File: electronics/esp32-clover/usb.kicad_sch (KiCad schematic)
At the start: 23 parts, among them J1 USB4055-30-A, Q2 MMDT3904, U2 CP2102N-Axx-xQFN20

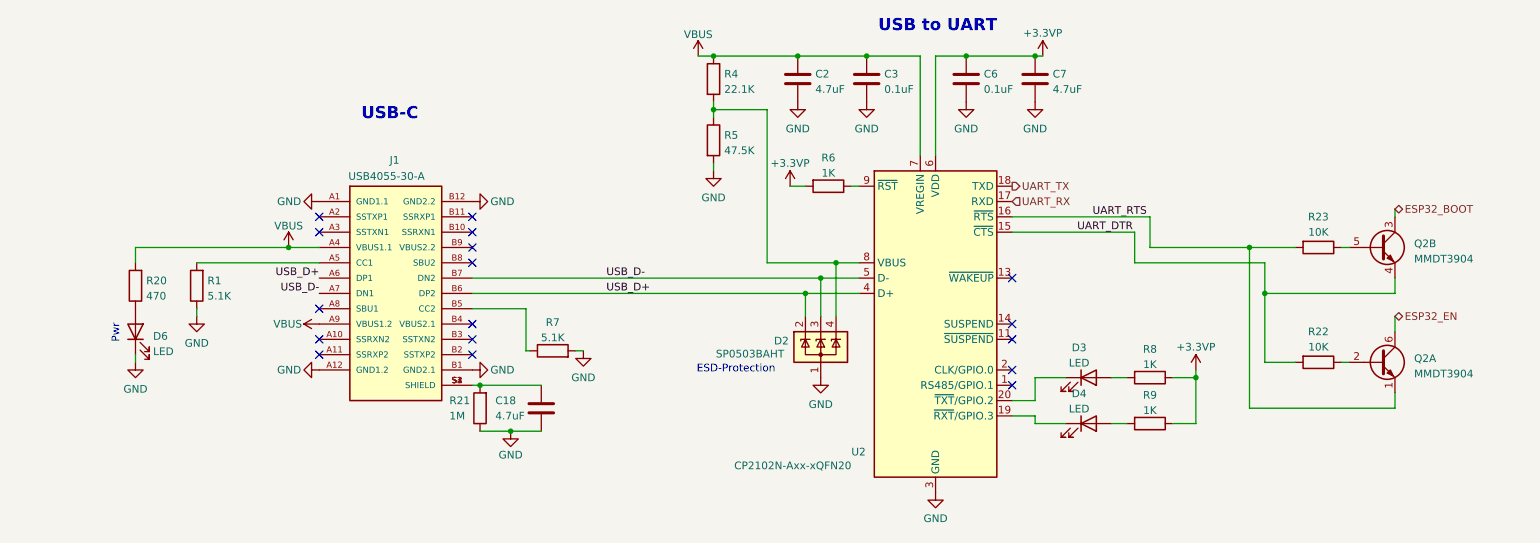
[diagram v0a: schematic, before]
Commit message: update before switching to stm32
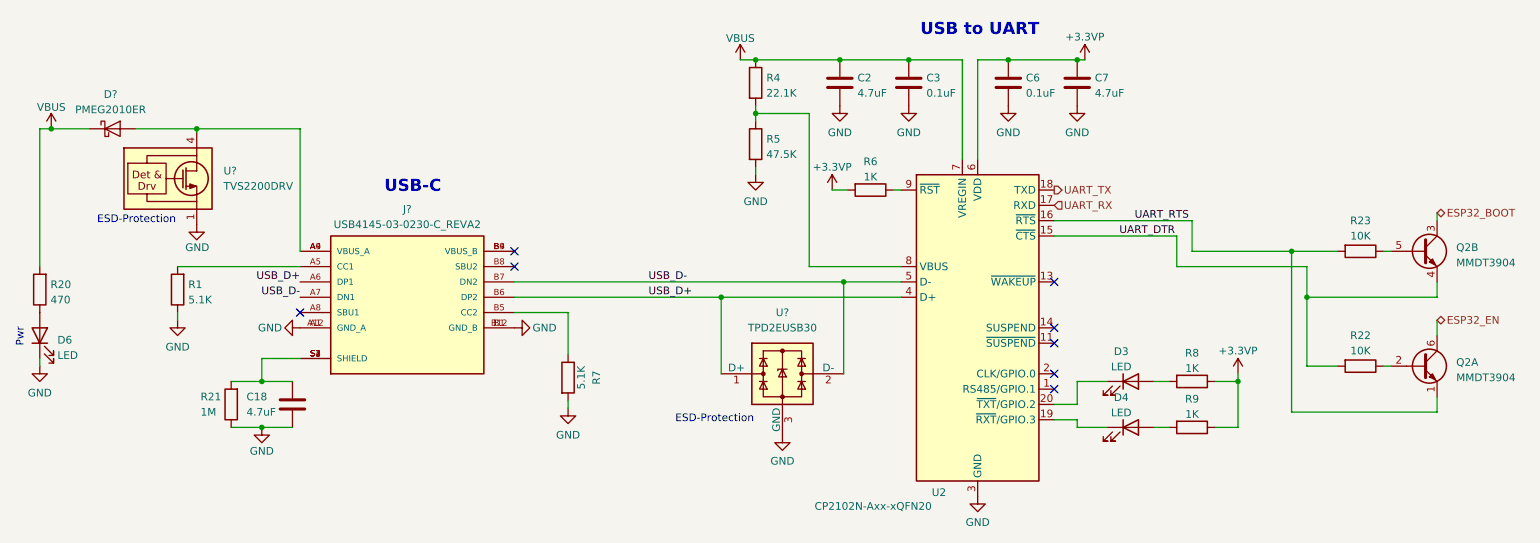
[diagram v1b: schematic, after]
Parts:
- removed D2: SP0503BAHT, Package_TO_SOT_SMD:SOT-143, symbol Power_Protection:SP0503BAHT
- removed J1: USB4055-30-A, USB4055-30-A:USB4055-30-A, symbol USB4055-30-A:USB4055-30-A
- added D?: PMEG2010ER, Diode_SMD:Nexperia_CFP3_SOD-123W, symbol Diode:PMEG2010ER
- added J?: USB4145-03-0230-C_REVA2, connectors_usb:USB4145-03-0230-C_REVA2, symbol connectors_usb:USB4145-03-0230-C_REVA2
- added U?: TVS2200DRV, Package_SON:WSON-6-1EP_2x2mm_P0.65mm_EP1x1.6mm, symbol Power_Protection:TVS2200DRV
- added U?: TPD2EUSB30, Package_TO_SOT_SMD:Texas_DRT-3, symbol Power_Protection:TPD2EUSB30
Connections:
- net GND: now also J?.A1 (GND_A), J?.A12 (GND_A), J?.B1 (GND_B), J?.B12 (GND_B), U?.1 (GND), U?.2 (GND), U?.3 (GND), U?.3 (GND), U?.7 (GND)
- net USB_D+: now also J?.A6 (DP1), J?.B6 (DP2), U?.1 (D+)
- net USB_D-: now also J?.A7 (DN1), J?.B7 (DN2), U?.2 (D-)
- net VBUS: now also D?.1 (K)
- net at C18.1, R21.2: now also J?.S1 (SHIELD), J?.S2 (SHIELD), J?.S3 (SHIELD), J?.S4 (SHIELD)
- net at R1.2: now also J?.A5 (CC1)
- net at R7.1: now also J?.B5 (CC2)
- new net: D?.2 (A), J?.A4 (VBUS_A), J?.A9 (VBUS_A), U?.4 (IN), U?.5 (IN), U?.6 (IN)
- new net: J?.B4 (VBUS_B), J?.B9 (VBUS_B)
- no-connect marks 17 -> 8
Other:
- moved on the sheet: C18, C2, C3, C6, C7, D3, D4, D6, Q2A, Q2B, R1, R20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
